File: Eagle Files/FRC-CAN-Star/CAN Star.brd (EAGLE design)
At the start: 51.5 x 30.7 mm, 12 parts

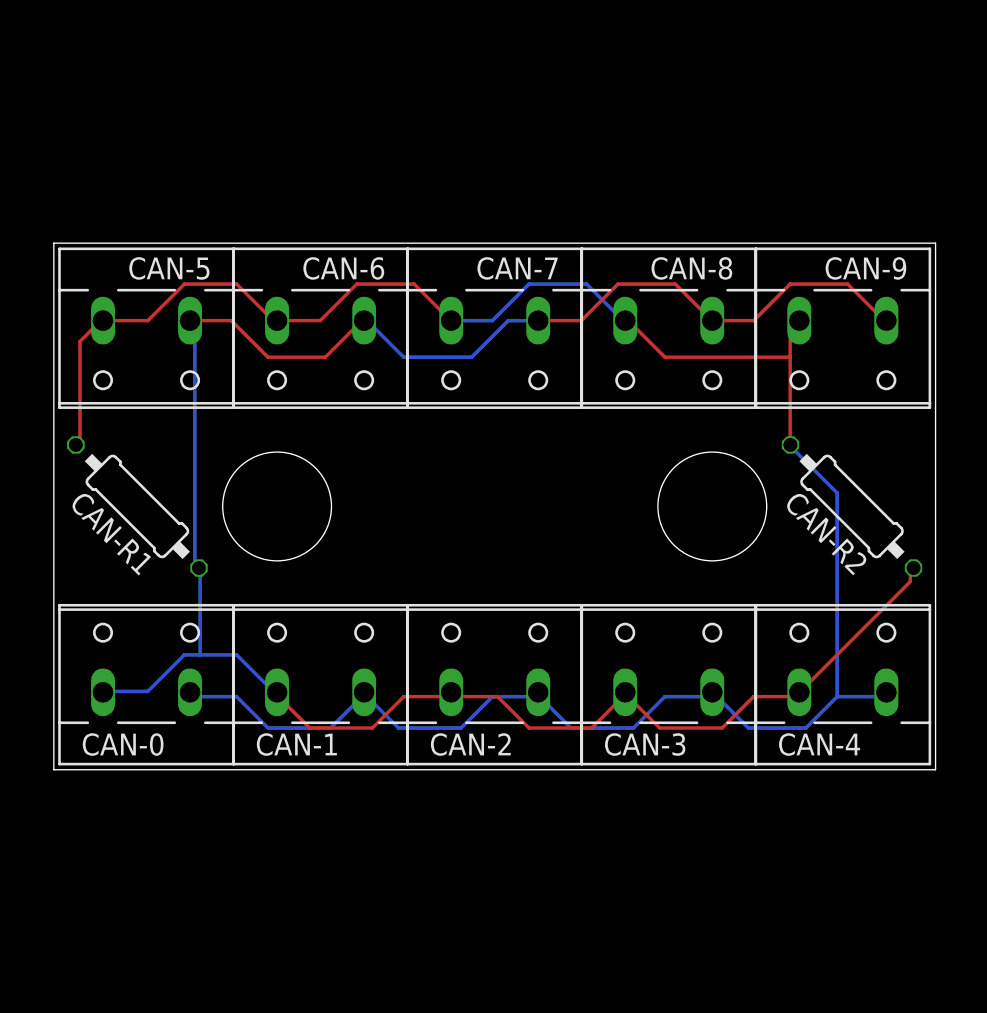
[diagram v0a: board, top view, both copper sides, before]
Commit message: Updated Eagle Files
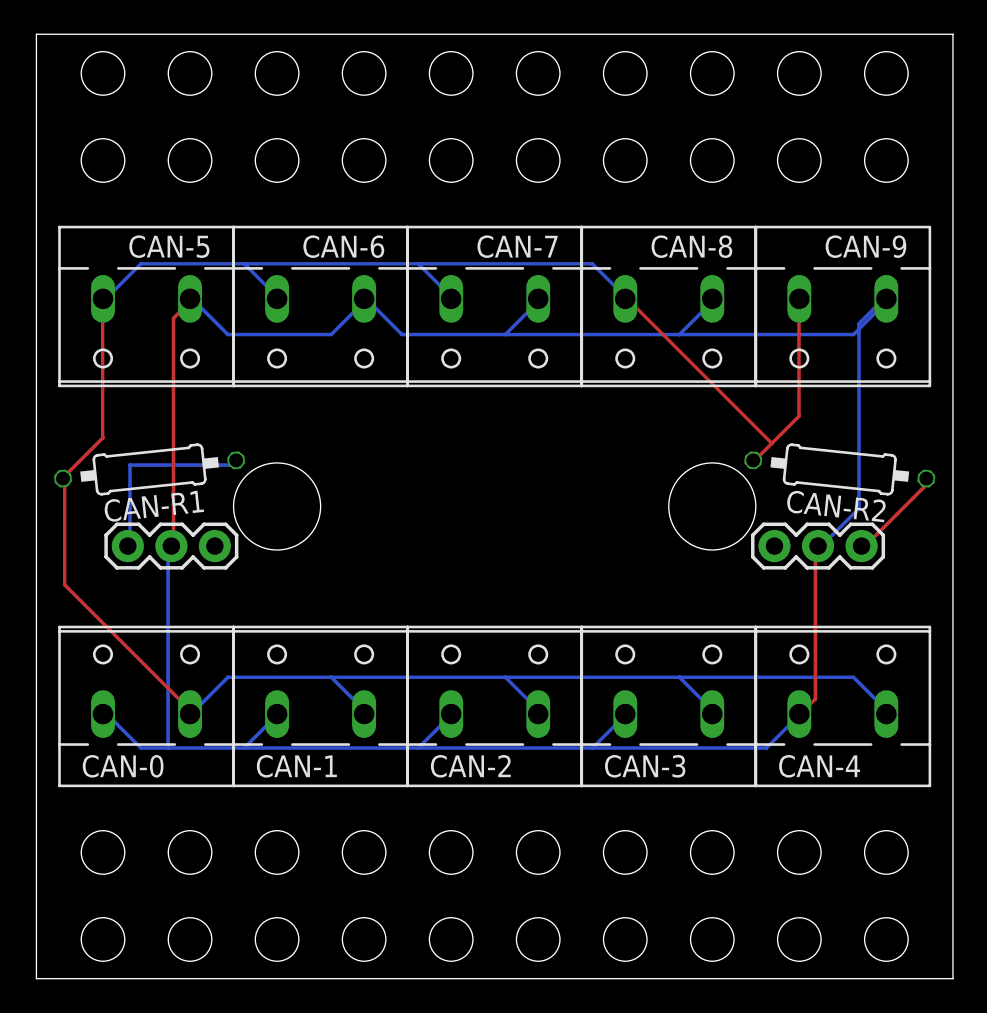
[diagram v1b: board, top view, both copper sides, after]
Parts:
- added JUMPER1, JUMPER2: (no value), SparkFun-Connectors:1X03
- moved CAN-R1 2.27 mm to (5.59, 17.5), turned to 186 degrees
- moved CAN-R2 2.27 mm to (45.9, 17.5), turned to 174 degrees
- moved CAN-0 1.27 mm to (5.41, 3.89)
- moved CAN-1 1.27 mm to (15.6, 3.89)
- moved CAN-2 1.27 mm to (25.7, 3.89)
- moved CAN-3 1.27 mm to (35.9, 3.89)
- moved CAN-4 1.27 mm to (46.1, 3.89)
- moved CAN-5 1.27 mm to (5.41, 26.8)
- moved CAN-6 1.27 mm to (15.6, 26.8)
- moved CAN-7 1.27 mm to (25.7, 26.8)
- moved CAN-8 1.27 mm to (35.9, 26.8)
- moved CAN-9 1.27 mm to (46.1, 26.8)
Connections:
- new net N$1: CAN-R1.1, JUMPER1.1
- new net N$2: CAN-R2.1, JUMPER2.1
- net CAN-A: now also JUMPER1.2, JUMPER2.2; no longer CAN-R1.1, CAN-R2.1
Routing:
- net CAN-A: track 125.6 -> 154.0 mm
- net CAN-B: track 125.6 -> 140.1 mm
- net N$1: track 0.00 -> 11.4 mm
- net N$2: track 0.00 -> 5.55 mm
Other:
- board size 51.5 x 30.7 mm -> 53.5 x 55.1 mm
- board text added: "G(L)"
- board text added: "ON"
- board text added: "Star Board v3"
- board text added: "Y(H)"
- board text removed: "Star Board v1"
